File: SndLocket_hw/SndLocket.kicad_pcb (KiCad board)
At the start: 2 copper layers, 44.9 x 138.8 mm, 0 parts

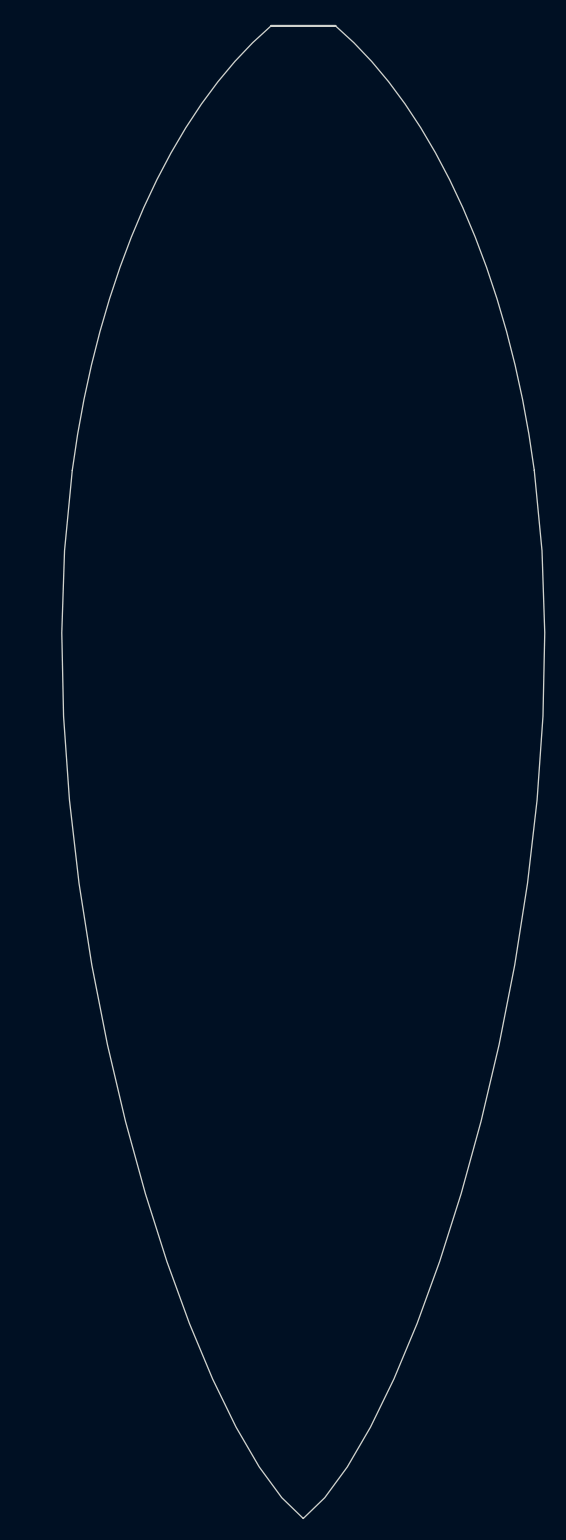
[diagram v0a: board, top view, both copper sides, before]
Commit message: .
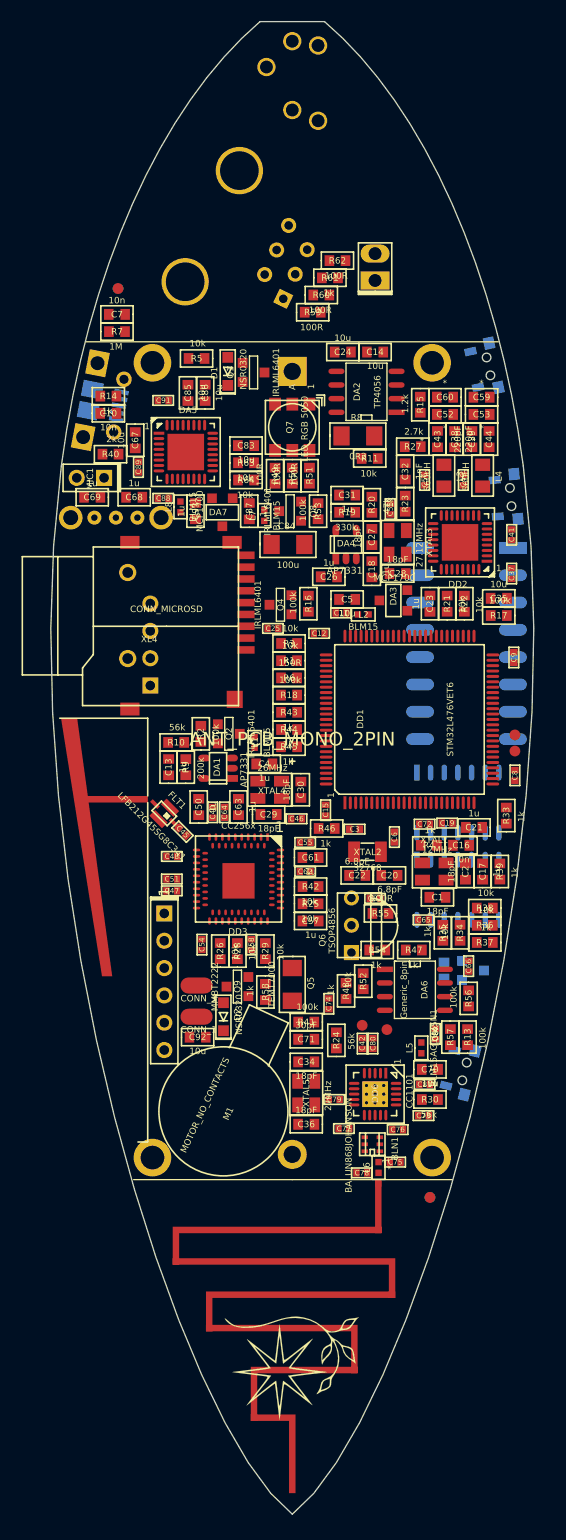
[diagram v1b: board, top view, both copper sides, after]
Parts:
- added ANT1: ANT_GENERAL, Antennas:LcktSnd_2d41, F.Cu at (147.4, 100.8)
- added ANT2: ANT_PCB_MONO_2PIN, Antennas:LcktSnd_868, F.Cu at (147.4, 139.8)
- added B1: BAT, Installation:18650x1, B.Cu at (147.4, 101.0)
- added BLN1: BALUN868JOHANSON, Radio:BALUN_JOHANSON868, F.Cu at (154.8, 136.5)
- added C1: 18pF, Capacitors:CAP_0603, F.Cu at (160.9, 113.5)
- added C10: 10n, Capacitors:CAP_0603, F.Cu at (130.3, 68.5)
- added C11: 0.1u, Capacitors:CAP_0402, F.Cu at (151.9, 87.1)
- added C12: 0.1u, Capacitors:CAP_0402, F.Cu at (149.9, 89.0)
- added C13: 1u, Capacitors:CAP_0603, F.Cu at (135.9, 101.4)
- added C14: 10u, Capacitors:CAP_0603, F.Cu at (155.1, 62.8)
- added C15: 0.1u, Capacitors:CAP_0402, F.Cu at (150.5, 105.4)
- added C16: 10n, Capacitors:CAP_0603, F.Cu at (163.1, 108.7)
- added C17: 1u, Capacitors:CAP_0603, F.Cu at (165.1, 111.1)
- added C18: 1u, Capacitors:CAP_0603, F.Cu at (154.8, 83.0)
- added C19: 0.1u, Capacitors:CAP_0402, F.Cu at (161.8, 106.6)
- added C2: 18pF, Capacitors:CAP_0603, F.Cu at (163.5, 111.1)
- added C20: 6.8pF, Capacitors:CAP_0603, F.Cu at (156.4, 111.5)
- added C21: 1u, Capacitors:CAP_0603, F.Cu at (164.3, 107.0)
- added C22: 6.8pF, Capacitors:CAP_0603, F.Cu at (153.4, 111.5)
- added C23: 1u, Capacitors:CAP_0603, F.Cu at (160.2, 86.2)
- added C24: 10u, Capacitors:CAP_0603, F.Cu at (152.1, 62.8)
- added C25: 0.1u, Capacitors:CAP_0402, F.Cu at (145.6, 88.5)
- added C26: 1u, Capacitors:CAP_0603, F.Cu at (150.8, 83.7)
- added C27: 18pF, Capacitors:CAP_0603, F.Cu at (154.8, 80.0)
- added C28: 18pF, Capacitors:CAP_0603, F.Cu at (157.2, 83.4)
- added C29: 18pF, Capacitors:CAP_0603, F.Cu at (145.2, 105.8)
- added C3: 0.1u, Capacitors:CAP_0402, F.Cu at (153.2, 107.2)
- added C30: 18pF, Capacitors:CAP_0603, F.Cu at (148.2, 103.5)
- added C31: 1u, Capacitors:CAP_0603, F.Cu at (152.5, 76.1)
- added C32: 1nF, Capacitors:CAP_0603, F.Cu at (157.9, 73.9)
- added C33: 0.1u, Capacitors:CAP_0402, F.Cu at (156.5, 77.4)
- added C34: 18pF, Capacitors:CAP_0603, F.Cu at (148.7, 128.8)
- added C35: 10u, Capacitors:CAP_0603, F.Cu at (166.6, 85.7)
- added C36: 18pF, Capacitors:CAP_0603, F.Cu at (148.7, 134.6)
- added C37: 0.1u, Capacitors:CAP_0402, F.Cu at (167.8, 83.4)
- added C38: 220pF, Capacitors:CAP_0603, F.Cu at (162.5, 70.9)
- added C39: 220pF, Capacitors:CAP_0603, F.Cu at (164.1, 70.9)
- added C4: 1u, Capacitors:CAP_0603, F.Cu at (144.8, 101.1)
- added C40: 0.1u, Capacitors:CAP_0402, F.Cu at (140.0, 105.6)
- added C41: 0.1u, Capacitors:CAP_0402, F.Cu at (167.8, 79.8)
- added C42: 0.1u, Capacitors:CAP_0402, F.Cu at (153.9, 127.1)
- added C43: *, Capacitors:CAP_0603, F.Cu at (160.9, 70.9)
- added C44: *, Capacitors:CAP_0603, F.Cu at (165.7, 70.9)
- added C45: 22pF, Capacitors:CAP_0402, F.Cu at (137.2, 107.4)
- added C46: 0.1u, Capacitors:CAP_0402, F.Cu at (147.8, 106.2)
- added C47: 0.1u, Capacitors:CAP_0402, F.Cu at (136.2, 112.9)
- added C48: 0.1u, Capacitors:CAP_0402, F.Cu at (136.2, 109.7)
- added C49: 0.1u, Capacitors:CAP_0402, F.Cu at (163.3, 74.7)
- added C5: 10u, Capacitors:CAP_0603, F.Cu at (152.5, 85.8)
- added C50: 1u, Capacitors:CAP_0603, F.Cu at (138.7, 105.1)
- added C51: 0.1u, Capacitors:CAP_0402, F.Cu at (136.2, 111.8)
- added C52: *, Capacitors:CAP_0603, F.Cu at (161.6, 68.6)
- added C53: *, Capacitors:CAP_0603, F.Cu at (165.0, 68.6)
- added C54: 0.1u, Capacitors:CAP_0402, F.Cu at (139.0, 117.9)
- added C55: 0.1u, Capacitors:CAP_0402, F.Cu at (148.6, 108.4)
- added C56: 0.1u, Capacitors:CAP_0402, F.Cu at (159.7, 74.7)
- added C57: 1u, Capacitors:CAP_0603, F.Cu at (149.1, 115.7)
- added C58: 0.1u, Capacitors:CAP_0402, F.Cu at (143.6, 117.9)
- added C59: *, Capacitors:CAP_0603, F.Cu at (165.0, 67.0)
- added C6: 0.1u, Capacitors:CAP_0402, F.Cu at (156.9, 107.9)
- added C60: *, Capacitors:CAP_0603, F.Cu at (161.6, 67.0)
- added C61: 1u, Capacitors:CAP_0603, F.Cu at (149.1, 109.8)
- added C62: 0.1u, Capacitors:CAP_0402, F.Cu at (148.6, 111.1)
- added C63: 1u, Capacitors:CAP_0603, F.Cu at (142.4, 105.1)
- added C64: 0.1u, Capacitors:CAP_0402, F.Cu at (141.1, 105.6)
- added C65: 0.1u, Capacitors:CAP_0402, F.Cu at (159.6, 115.6)
- added C66: 0.1u, Capacitors:CAP_0402, F.Cu at (163.8, 119.9)
- added C67: 10u, Capacitors:CAP_0603, F.Cu at (132.8, 71.0)
- added C68: 1u, Capacitors:CAP_0603, F.Cu at (132.7, 76.3)
- added C69: 1u, Capacitors:CAP_0603, F.Cu at (128.8, 76.3)
- added C7: 10n, Capacitors:CAP_0603, F.Cu at (131.1, 59.3)
- added C70: 10u, Capacitors:CAP_0603, F.Cu at (160.2, 129.5)
- added C71: 30pF, Capacitors:CAP_0603, F.Cu at (148.7, 126.7)
- added C72: 0.1u, Capacitors:CAP_0402, F.Cu at (159.7, 106.7)
- added C73: 0.1u, Capacitors:CAP_0402, F.Cu at (159.6, 133.8)
- added C74: 0.1u, Capacitors:CAP_0402, F.Cu at (150.8, 123.4)
- added C75: *, Capacitors:CAP_0402, F.Cu at (157.0, 138.1)
- added C76: 0.1u, Capacitors:CAP_0402, F.Cu at (157.2, 135.1)
- added C77: 0.1u, Capacitors:CAP_0402, F.Cu at (152.2, 135.0)
- added C78: *, Capacitors:CAP_0402, F.Cu at (153.9, 139.1)
- added C79: 0.1u, Capacitors:CAP_0402, F.Cu at (151.3, 132.3)
- added C8: 0.1u, Capacitors:CAP_0402, F.Cu at (168.1, 102.2)
- added C80: 0.1u, Capacitors:CAP_0402, F.Cu at (154.9, 127.1)
- added C81: 0.1u, Capacitors:CAP_0402, F.Cu at (159.7, 130.9)
- added C82: 0.1u, Capacitors:CAP_0402, F.Cu at (155.1, 113.6)
- added C83: 10u, Capacitors:CAP_0603, F.Cu at (143.1, 71.5)
- added C84: 100u, Capacitors:CAP_1206, F.Cu at (147.0, 80.7)
- added C85: 10u, Capacitors:CAP_0603, F.Cu at (137.7, 66.6)
- added C86: 10u, Capacitors:CAP_0603, F.Cu at (139.3, 66.6)
- added C87: 1u, Capacitors:CAP_0603, F.Cu at (143.4, 77.6)
- added C88: 0.1u, Capacitors:CAP_0402, F.Cu at (135.4, 76.4)
- added C89: 0.1u, Capacitors:CAP_0402, F.Cu at (133.1, 73.5)
- added C9: 0.1u, Capacitors:CAP_0402, F.Cu at (168.0, 91.2)
- added C90: 0.1u, Capacitors:CAP_0402, F.Cu at (160.7, 126.2)
- added C91: 0.1u, Capacitors:CAP_0402, F.Cu at (135.4, 67.3)
- added C92: 10u, Capacitors:CAP_0603, F.Cu at (138.6, 126.5)
- added C93: 1u, Capacitors:CAP_0603, F.Cu at (138.4, 77.6)
- added D1: NSR0320, Diodes:SOD323, F.Cu at (141.4, 64.6)
- added D2: NSR0320, Diodes:SOD323, F.Cu at (141.0, 124.6)
- added DA1: AP7331, SOT:SOT23-5, F.Cu at (140.5, 101.5)
- added DA2: TP4056, SO_DIL_TSSOP:SO8_150MIL, F.Cu at (154.3, 66.5)
- added DA3: MCP1700, SOT:SOT23-3A, F.Cu at (156.8, 85.9)
- added DA4: AP7331, SOT:SOT23-5, F.Cu at (152.4, 80.7)
- added DA5: WM8960, QFN_DFN:QFN32_EP_5x5_Pitch0.5mm, F.Cu at (137.5, 72.1)
- added DA6: Generic_8pin, SO_DIL_TSSOP:SO8_150MIL, F.Cu at (158.8, 122.1)
- added DA7: MCP1700, SOT:SOT23-3A, F.Cu at (140.9, 77.7)
- added DD1: STM32L476VET6, LQFP_TQFP:LQFP100, F.Cu at (158.3, 97.0)
- added DD2: MFRC52202, QFN_DFN:QFN32_EP_5x5_Pitch0.5mm, F.Cu at (163.0, 80.5)
- added DD3: CC256x, QFN_DFN:mrQFN76, F.Cu at (142.4, 111.8)
- added DD4: SN74LVC07, SO_DIL_TSSOP:SO14, B.Cu at (162.8, 104.7)
- added DD5: SN74LVC07, SO_DIL_TSSOP:SO14, B.Cu at (162.8, 112.8)
- added DD6: CC1101, QFN_DFN:QFN20, F.Cu at (155.1, 131.8)
- added FLT1: LFB212G45SG8C341, Radio:FLT_LFB21, F.Cu at (135.5, 105.7)
- added HOLE1: HOLE_METALLED, PCB:Hole2d2_out3d5mm, F.Cu at (134.4, 137.7)
- added HOLE2: HOLE_METALLED, PCB:Hole2d2_out3d5mm, F.Cu at (160.4, 137.7)
- added HOLE3: HOLE_METALLED, PCB:Hole2d2_out3d5mm, F.Cu at (134.4, 63.8)
- added HOLE4: HOLE_METALLED, PCB:Hole2d2_out3d5mm, F.Cu at (160.4, 63.8)
- added L1: BLM15, Inductors:IND_0402, F.Cu at (143.9, 99.1)
- added L2: BLM15, Inductors:IND_0402, F.Cu at (154.0, 87.2)
- added L3: 560nH, Inductors:IND_0805, F.Cu at (161.5, 74.3)
- added L4: 560nH, Inductors:IND_0805, F.Cu at (165.1, 74.3)
- added L5: BLM15AG102SN1, Inductors:IND_0402, F.Cu at (159.4, 127.5)
- added L6: *, Inductors:IND_0402, F.Cu at (155.4, 138.6)
- added L7: BLM15, Inductors:IND_0402, F.Cu at (144.8, 78.0)
- added L8: BLM15, Inductors:IND_0402, F.Cu at (137.0, 77.2)
- added Logo1: Logo, Pictures:Ostranna_12d7_10d1, F.Cu at (147.4, 157.3)
- added M1: MOTOR_NO_CONTACTS, Installation:Motor_no_Contacts, F.Cu at (141.0, 133.4)
- added MIC1: Microphone, Connectors:PLS-2, F.Cu at (129.9, 74.5)
- added Q1: IRLML6401, SOT:SOT23-3, F.Cu at (143.8, 64.7)
- added Q2: IRLML6401, SOT:SOT23-3, F.Cu at (141.5, 98.3)
- added Q3: IRLML6401, SOT:SOT23-3, B.Cu at (164.2, 120.3)
- added Q4: IRLML6401, SOT:SOT23-3, F.Cu at (146.3, 86.3)
- added Q5: TEMT7000, Resistors:RES_1206, F.Cu at (147.4, 121.6)
- added Q6: TSOP4856, Sensors:TSOP48xx, F.Cu at (152.9, 116.1)
- added Q7: LED_RGB 5050, LEDs:LED_5050, F.Cu at (147.4, 69.8)
- added Q8: IRLML6401, SOT:SOT23-3, F.Cu at (147.2, 77.6)
- added Q9: MMBT2222, SOT:SOT23-3, F.Cu at (142.3, 121.8)
- added R1: 10k, Resistors:RES_0603, F.Cu at (147.1, 91.5)
- added R10: 56k, Resistors:RES_0603, F.Cu at (136.6, 99.1)
- added R11: 10k, Resistors:RES_0603, F.Cu at (154.6, 72.7)
- added R12: 100k, Resistors:RES_0603, B.Cu at (161.5, 120.3)
- added R13: 100k, Resistors:RES_0603, F.Cu at (163.7, 126.5)
- added R14: 1k, Resistors:RES_0603, F.Cu at (130.3, 66.9)
- added R15: 1.2k, Resistors:RES_0603, F.Cu at (159.3, 67.7)
- added R16: 100k, Resistors:RES_0603, F.Cu at (148.9, 86.2)
- added R17: 100k, Resistors:RES_0603, F.Cu at (166.6, 87.3)
- added R18: 100k, Resistors:RES_0603, F.Cu at (147.1, 94.7)
- added R19: 330k, Resistors:RES_0603, F.Cu at (152.5, 77.7)
- added R2: 100k, Resistors:RES_0603, F.Cu at (138.9, 98.3)
- added R20: 47k, Resistors:RES_0603, F.Cu at (154.8, 77.0)
- added R21: 10k, Resistors:RES_0603, F.Cu at (161.8, 86.2)
- added R22: 10k, Resistors:RES_0603, F.Cu at (163.4, 86.2)
- added R23: 1k, Resistors:RES_0603, F.Cu at (157.9, 76.9)
- added R24: 56k, Resistors:RES_0603, F.Cu at (151.5, 126.8)
- added R25: 10k, Resistors:RES_0603, F.Cu at (149.1, 114.1)
- added R26: 10k, Resistors:RES_0603, F.Cu at (140.7, 118.5)
- added R27: 2.7k, Resistors:RES_0603, F.Cu at (158.6, 71.6)
- added R28: 10k, Resistors:RES_0603, F.Cu at (142.3, 118.5)
- added R29: 10k, Resistors:RES_0603, F.Cu at (144.9, 118.5)
- added R3: 10k, Resistors:RES_0603, F.Cu at (147.1, 89.9)
- added R30: 56k, Resistors:RES_0603, F.Cu at (160.2, 132.3)
- added R33: 1k, Resistors:RES_0603, F.Cu at (167.3, 105.9)
- added R34: 10k, Resistors:RES_0603, F.Cu at (163.0, 116.8)
- added R35: 1k, Resistors:RES_0603, F.Cu at (161.4, 116.8)
- added R36: 10k, Resistors:RES_0603, F.Cu at (165.3, 116.1)
- added R37: 1k, Resistors:RES_0603, F.Cu at (165.3, 117.7)
- added R38: 10k, Resistors:RES_0603, F.Cu at (165.3, 114.5)
- added R39: 1k, Resistors:RES_0603, F.Cu at (166.7, 111.1)
- added R4: 1k, Resistors:RES_0603, F.Cu at (160.1, 108.7)
- added R40: 2k, Resistors:RES_0603, F.Cu at (130.5, 72.3)
- added R41: 100k, Resistors:RES_0603, F.Cu at (148.7, 125.1)
- added R42: 10k, Resistors:RES_0603, F.Cu at (149.1, 112.5)
- added R43: 1k, Resistors:RES_0603, F.Cu at (147.1, 96.3)
- added R44: 1k, Resistors:RES_0603, F.Cu at (147.1, 97.9)
- added R45: 1k, Resistors:RES_0603, F.Cu at (147.1, 99.5)
- added R46: 1k, Resistors:RES_0603, F.Cu at (150.6, 107.1)
- added R47: 1k, Resistors:RES_0603, F.Cu at (158.7, 118.4)
- added R48: 1k, Resistors:RES_0603, F.Cu at (152.4, 122.2)
- added R49: 100R, Resistors:RES_0603, F.Cu at (145.8, 74.3)
- added R5: 10k, Resistors:RES_0603, F.Cu at (138.5, 63.4)
- added R50: 100R, Resistors:RES_0603, F.Cu at (147.4, 74.3)
- added R51: 100R, Resistors:RES_0603, F.Cu at (149.0, 74.3)
- added R52: 10k, Resistors:RES_0603, F.Cu at (154.0, 121.3)
- added R53: 100k, Resistors:RES_0603, F.Cu at (149.8, 77.6)
- added R54: 1k, Resistors:RES_0603, F.Cu at (155.3, 118.4)
- added R55: 100R, Resistors:RES_0603, F.Cu at (155.6, 115.0)
- added R56: 100k, Resistors:RES_0603, F.Cu at (163.8, 122.9)
- added R57: 100k, Resistors:RES_0603, F.Cu at (162.1, 126.5)
- added R58: 1k, Resistors:RES_0603, F.Cu at (144.9, 122.3)
- added R59: 100R, Resistors:RES_0603, F.Cu at (149.3, 59.1)
- added R6: 150R, Resistors:RES_0603, F.Cu at (147.1, 93.1)
- added R60: 100R, Resistors:RES_0603, F.Cu at (150.1, 57.5)
- added R61: 1k, Resistors:RES_0603, F.Cu at (150.9, 55.9)
- added R62: 100R, Resistors:RES_0603, F.Cu at (151.6, 54.3)
- added R63: 10k, Resistors:RES_0603, F.Cu at (143.1, 73.1)
- added R64: 10k, Resistors:RES_0603, F.Cu at (143.1, 74.7)
- added R7: 1M, Resistors:RES_0603, F.Cu at (131.1, 60.9)
- added R8: 0R2, Resistors:RES_1206, F.Cu at (153.5, 70.6)
- added R9: 200k, Resistors:RES_0603, F.Cu at (137.5, 101.4)
- added RP1: REFPOINT, PCB:REF_POINT_1MM, B.Cu at (131.2, 56.9)
- added RP2: REFPOINT, PCB:REF_POINT_1MM, B.Cu at (160.2, 141.4)
- added RP3: REFPOINT, PCB:REF_POINT_1MM, F.Cu at (160.2, 141.4)
- added RP4: REFPOINT, PCB:REF_POINT_1MM, F.Cu at (131.2, 56.9)
- added SW1: SWITCH, BtnsSwitches:SW_SS-1P2T_Housing, B.Cu at (131.0, 78.2)
- added SW2: DIPx8, BtnsSwitches:DIP_SMD_X8, B.Cu at (163.6, 89.9)
- added SW3: BUTTON, BtnsSwitches:BTN_IT1198, B.Cu at (165.4, 130.2)
- added SW4: BUTTON, BtnsSwitches:BTN_IT1198, B.Cu at (169.8, 76.1)
- added SW5: BUTTON, BtnsSwitches:BTN_IT1198, B.Cu at (167.7, 63.7)
- added TP1: TESTPOINT, PCB:TESTPOINT_1MM, F.Cu at (168.1, 98.4)
- added TP10: TESTPOINT, PCB:TESTPOINT_1MM, F.Cu at (156.2, 125.8)
- added TP2: TESTPOINT, PCB:TESTPOINT_1MM, F.Cu at (168.1, 99.9)
- added TP9: TESTPOINT, PCB:TESTPOINT_1MM, F.Cu at (153.9, 125.4)
- added XL1: CONN_4, Connectors:PBS-4R, B.Cu at (134.2, 90.0)
- added XL2: USB_MICRO, Connectors:USBmicro_MOLEX_1050170001, B.Cu at (127.2, 67.0)
- added XL3: CONN_6, Connectors:PLS-6, B.Cu at (135.5, 115.0)
- added XL4: CONN_MICROSD, Installation:MICROSD_EJECTOR_TFWF1, F.Cu at (142.3, 88.3)
- added XL5: AudioJackSimple, Connectors:AUDIO_CKX3_5_30, B.Cu at (147.4, 32.1)
- added XL6: CONN_1, PCB:Oval3x1.5, F.Cu at (138.5, 124.6)
- added XL7: CONN_1, PCB:Oval3x1.5, F.Cu at (138.5, 121.7)
- added XL8: RJ12, Connectors:RJ11_TJ6_6P6C, B.Cu at (133.4, 47.9)
- added XL9: CONN_2, Connectors:SLD_2_2D5, F.Cu at (155.1, 54.9)
- added XTAL1: 12MHz, Quartz:03225C4, F.Cu at (160.6, 111.1)
- added XTAL2: 32768, Quartz:03215C2, F.Cu at (154.4, 109.3)
- added XTAL3: 27.12MHz, Quartz:03225C4, F.Cu at (157.2, 80.5)
- added XTAL4: 26MHz, Quartz:03225C4, F.Cu at (145.3, 103.5)
- added XTAL5: 27MHz, Quartz:03225C4, F.Cu at (148.7, 131.7)
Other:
- copper layers 2 -> 4
- net class Default: clearance 0.2 -> 0.16; trace_width 0.25 -> 0.16; via_dia 0.8 -> 0.7; via_drill 0.4 -> 0.3
- net class Wide added: clearance 0.2, trace_width 0.5, via_dia 0.7, via_drill 0.3
- rule trace_clearance: 0.2 -> 0.16
- rule trace_min: 0.2 -> 0.1
